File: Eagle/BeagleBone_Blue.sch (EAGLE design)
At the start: 138 parts, among them M1 JST_ZH_2, M2 JST_ZH_2, M3 JST_ZH_2, M4 JST_ZH_2, Q3 MOSFET-N, U1 OSD3358

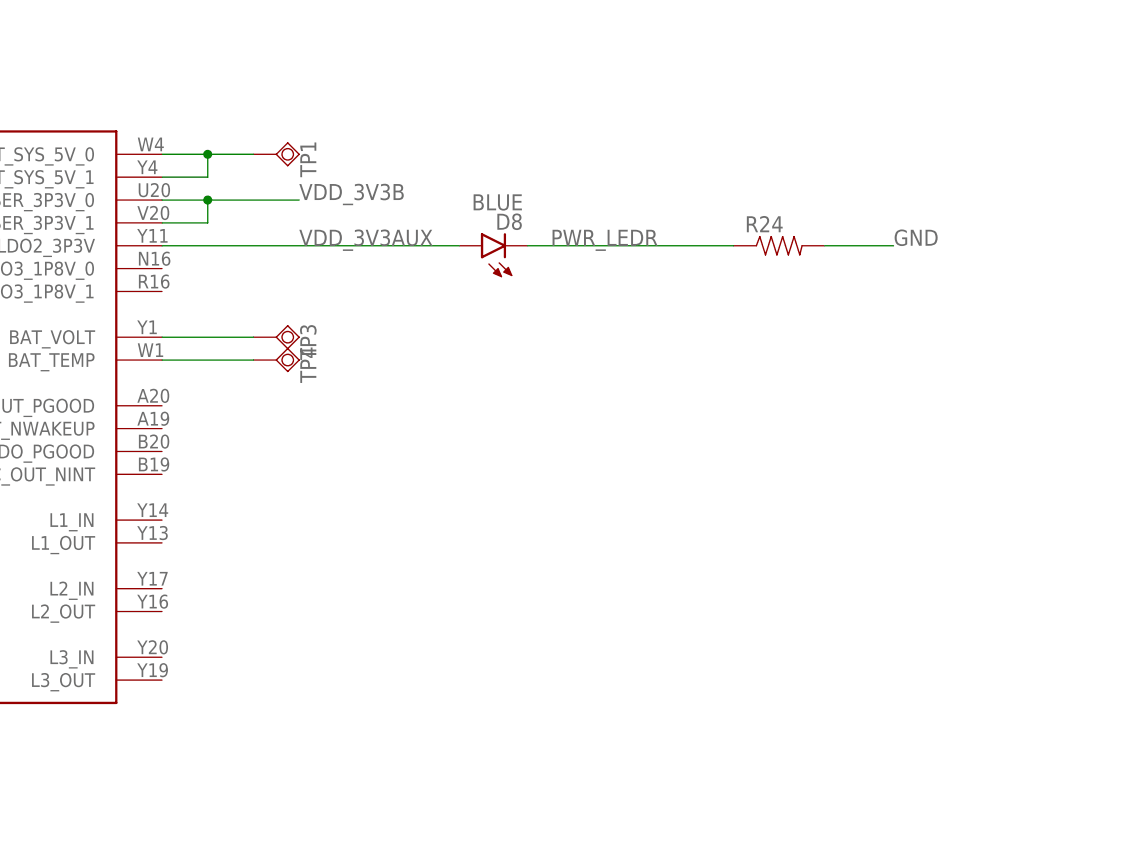
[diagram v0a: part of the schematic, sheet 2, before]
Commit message: Finished SIP-A
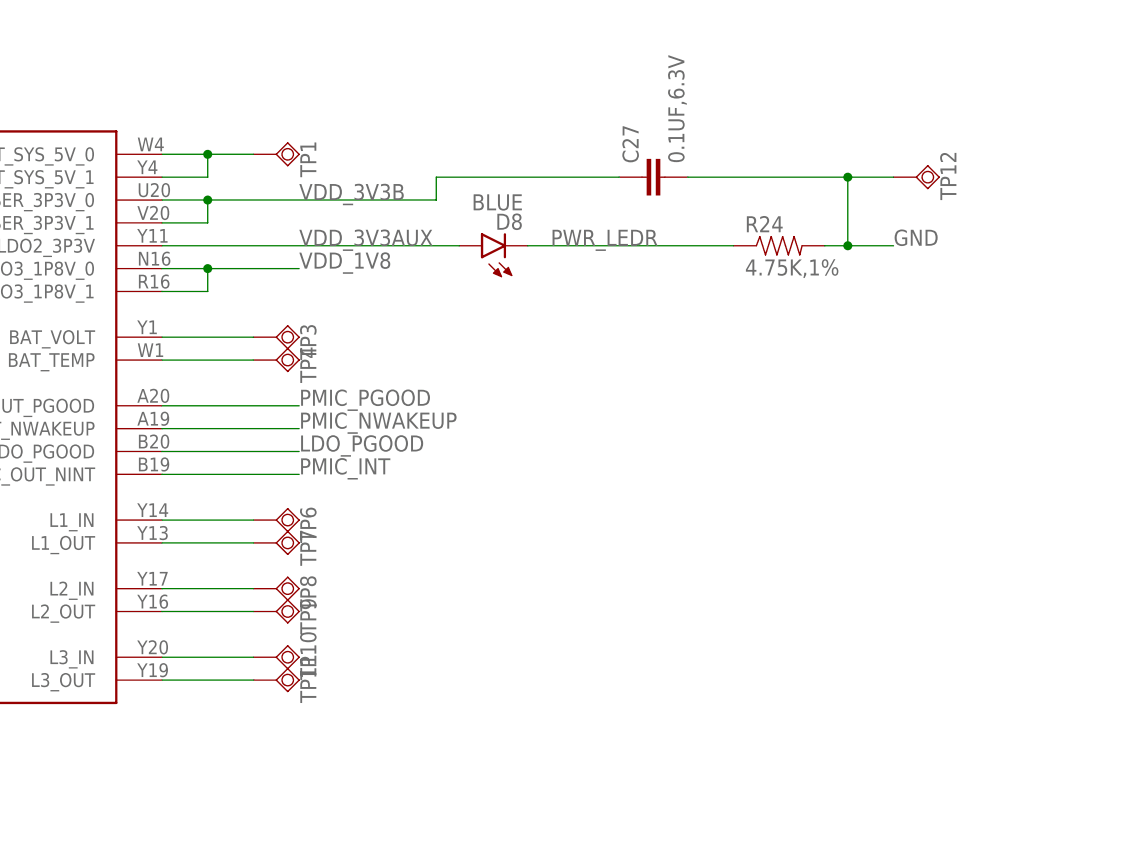
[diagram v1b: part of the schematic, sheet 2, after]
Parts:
- added C27: 0.1UF,6.3V, Strawson_Eagle_Lib:CAP0402-CAP
- added TP10, TP11, TP12, TP6, TP7, TP8, TP9: TPSQB1,27, testpad:TPSQB1,27
- R24: value (none) -> 4.75K,1%
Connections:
- new net LDO_PGOOD: U1A.PMIC_OUT_LDO_PGOOD
- new net N$13: TP6.TP, U1A.L1_IN
- new net N$19: TP7.TP, U1A.L1_OUT
- new net N$20: TP8.TP, U1A.L2_IN
- new net N$21: TP9.TP, U1A.L2_OUT
- new net N$22: TP10.TP, U1A.L3_IN
- new net N$23: TP11.TP, U1A.L3_OUT
- new net PMIC_INT: U1A.PMIC_OUT_NINT
- new net PMIC_NWAKEUP: U1A.PMIC_OUT_NWAKEUP
- new net PMIC_PGOOD: U1A.PMIC_OUT_PGOOD
- new net VDD_1V8: U1A.VOUT_LDO3_1P8V_0, U1A.VOUT_LDO3_1P8V_1
- net GND: now also C27.2, TP12.TP
- net VDD_3V3B: now also C27.1
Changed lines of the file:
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@@
 <part name="R23" library="Strawson_Eagle_Lib" deviceset="RESISTOR" device="0402-RES" value="1.5K,1%"/>
 <part name="D8" library="BeagleBone_Blue" deviceset="LED" device="0603" value="BLUE"/>
-<part name="R24" library="Strawson_Eagle_Lib" deviceset="RESISTOR" device="0402-RES"/>
+<part name="R24" library="Strawson_Eagle_Lib" deviceset="RESISTOR" device="0402-RES" value="4.75K,1%"/>
+<part name="TP6" library="testpad" deviceset="TPSQ" device="B1,27"/>
+<part name="TP7" library="testpad" deviceset="TPSQ" device="B1,27"/>
+<part name="TP8" library="testpad" deviceset="TPSQ" device="B1,27"/>
+<part name="TP9" library="testpad" deviceset="TPSQ" device="B1,27"/>
+<part name="TP10" library="testpad" deviceset="TPSQ" device="B1,27"/>
+<part name="TP11" library="testpad" deviceset="TPSQ" device="B1,27"/>
+<part name="TP12" library="testpad" deviceset="TPSQ" device="B1,27"/>
+<part name="C27" library="Strawson_Eagle_Lib" deviceset="CAP" device="0402-CAP" value="0.1UF,6.3V"/>
 </parts>
 <sheets>
@@
 <instance part="D8" gate="G$1" x="160.02" y="238.76" rot="R90"/>
 <instance part="R24" gate="G$1" x="193.04" y="238.76"/>
+<instance part="TP6" gate="G$1" x="137.16" y="208.28" rot="R90"/>
+<instance part="TP7" gate="G$1" x="137.16" y="205.74" rot="R90"/>
+<instance part="TP8" gate="G$1" x="137.16" y="200.66" rot="R90"/>
+<instance part="TP9" gate="G$1" x="137.16" y="198.12" rot="R90"/>
+<instance part="TP10" gate="G$1" x="137.16" y="193.04" rot="R90"/>
+<instance part="TP11" gate="G$1" x="137.16" y="190.5" rot="R90"/>
+<instance part="TP12" gate="G$1" x="208.28" y="246.38" rot="R90"/>
+<instance part="C27" gate="G$1" x="180.34" y="246.38" rot="R90"/>
 </instances>
 <busses>
@@
 <wire x1="124.46" y1="243.84" x2="129.54" y2="243.84" width="0.1524" layer="91"/>
 <pinref part="U1" gate="A" pin="VOUT_USER_3P3V_1"/>
-<wire x1="129.54" y1="243.84" x2="139.7" y2="243.84" width="0.1524" layer="91"/>
 <wire x1="124.46" y1="241.3" x2="129.54" y2="241.3" width="0.1524" layer="91"/>
 <wire x1="129.54" y1="241.3" x2="129.54" y2="243.84" width="0.1524" layer="91"/>
 <junction x="129.54" y="243.84"/>
 <label x="139.7" y="243.84" size="1.778" layer="95"/>
+<wire x1="129.54" y1="243.84" x2="154.94" y2="243.84" width="0.1524" layer="91"/>
+<wire x1="154.94" y1="243.84" x2="154.94" y2="246.38" width="0.1524" layer="91"/>
+<pinref part="C27" gate="G$1" pin="1"/>
+<wire x1="154.94" y1="246.38" x2="175.26" y2="246.38" width="0.1524" layer="91"/>
 </segment>
 </net>
@@
 <segment>
 <pinref part="R24" gate="G$1" pin="2"/>
-<wire x1="198.12" y1="238.76" x2="205.74" y2="238.76" width="0.1524" layer="91"/>
+<wire x1="198.12" y1="238.76" x2="200.66" y2="238.76" width="0.1524" layer="91"/>
 <label x="205.74" y="238.76" size="1.778" layer="95"/>
-</segment>
-</net>
+<pinref part="TP12" gate="G$1" pin="TP"/>
+<pinref part="C27" gate="G$1" pin="2"/>
+<wire x1="182.88" y1="246.38" x2="200.66" y2="246.38" width="0.1524" layer="91"/>
+<wire x1="200.66" y1="246.38" x2="205.74" y2="246.38" width="0.1524" layer="91"/>
+<wire x1="205.74" y1="238.76" x2="200.66" y2="238.76" width="0.1524" layer="91"/>
+<wire x1="200.66" y1="238.76" x2="200.66" y2="246.38" width="0.1524" layer="91"/>
+<junction x="200.66" y="246.38"/>
+<junction x="200.66" y="238.76"/>
+</segment>
+</net>
+<net name="VDD_1V8" class="0">
+<segment>
+<pinref part="U1" gate="A" pin="VOUT_LDO3_1P8V_0"/>
+<wire x1="124.46" y1="236.22" x2="129.54" y2="236.22" width="0.1524" layer="91"/>
+<pinref part="U1" gate="A" pin="VOUT_LDO3_1P8V_1"/>
+<wire x1="129.54" y1="236.22" x2="139.7" y2="236.22" width="0.1524" layer="91"/>
+<wire x1="124.46" y1="233.68" x2="129.54" y2="233.68" width="0.1524" layer="91"/>
+<wire x1="129.54" y1="233.68" x2="129.54" y2="236.22" width="0.1524" layer="91"/>
+<junction x="129.54" y="236.22"/>
+<label x="139.7" y="236.22" size="1.778" layer="95"/>
+</segment>
+</net>
+<net name="PMIC_PGOOD" class="0">
+<segment>
+<pinref part="U1" gate="A" pin="PMIC_OUT_PGOOD"/>
+<wire x1="124.46" y1="220.98" x2="139.7" y2="220.98" width="0.1524" layer="91"/>
+<label x="139.7" y="220.98" size="1.778" layer="95"/>
+</segment>
+</net>
+<net name="PMIC_NWAKEUP" class="0">
+<segment>
+<pinref part="U1" gate="A" pin="PMIC_OUT_NWAKEUP"/>
+<wire x1="124.46" y1="218.44" x2="139.7" y2="218.44" width="0.1524" layer="91"/>
+<label x="139.7" y="218.44" size="1.778" layer="95"/>
+</segment>
+</net>
+<net name="LDO_PGOOD" class="0">
+<segment>
+<pinref part="U1" gate="A" pin="PMIC_OUT_LDO_PGOOD"/>
+<wire x1="124.46" y1="215.9" x2="139.7" y2="215.9" width="0.1524" layer="91"/>
+<label x="139.7" y="215.9" size="1.778" layer="95"/>
+</segment>
+</net>
+<net name="PMIC_INT" class="0">
+<segment>
+<pinref part="U1" gate="A" pin="PMIC_OUT_NINT"/>
+<wire x1="124.46" y1="213.36" x2="139.7" y2="213.36" width="0.1524" layer="91"/>
+<label x="139.7" y="213.36" size="1.778" layer="95"/>
+</segment>
+</net>
+<net name="N$13" class="0">
+<segment>
+<pinref part="U1" gate="A" pin="L1_IN"/>
+<pinref part="TP6" gate="G$1" pin="TP"/>
+<wire x1="124.46" y1="208.28" x2="134.62" y2="208.28" width="0.1524" layer="91"/>
+</segment>
+</net>
+<net name="N$19" class="0">
+<segment>
+<pinref part="U1" gate="A" pin="L1_OUT"/>
+<pinref part="TP7" gate="G$1" pin="TP"/>
+<wire x1="124.46" y1="205.74" x2="134.62" y2="205.74" width="0.1524" layer="91"/>
+</segment>
+</net>
+<net name="N$20" class="0">
+<segment>
+<pinref part="U1" gate="A" pin="L2_IN"/>
+<pinref part="TP8" gate="G$1" pin="TP"/>
+<wire x1="124.46" y1="200.66" x2="134.62" y2="200.66" width="0.1524" layer="91"/>
+</segment>
+</net>
+<net name="N$21" class="0">
+<segment>
+<pinref part="U1" gate="A" pin="L2_OUT"/>
+<pinref part="TP9" gate="G$1" pin="TP"/>
+<wire x1="124.46" y1="198.12" x2="134.62" y2="198.12" width="0.1524" layer="91"/>
+</segment>
+</net>
+<net name="N$22" class="0">
+<segment>
+<pinref part="U1" gate="A" pin="L3_IN"/>
+<pinref part="TP10" gate="G$1" pin="TP"/>
+<wire x1="124.46" y1="193.04" x2="134.62" y2="193.04" width="0.1524" layer="91"/>
+</segment>
+</net>
+<net name="N$23" class="0">
+<segment>
+<pinref part="U1" gate="A" pin="L3_OUT"/>
+<pinref part="TP11" gate="G$1" pin="TP"/>
+<wire x1="124.46" y1="190.5" x2="134.62" y2="190.5" width="0.1524" layer="91"/>
+</segment>
+</net>
